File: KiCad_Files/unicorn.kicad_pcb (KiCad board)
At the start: 2 copper layers, 50 x 49.9 mm, 8 parts, among them SW1 SW_DIP_x01

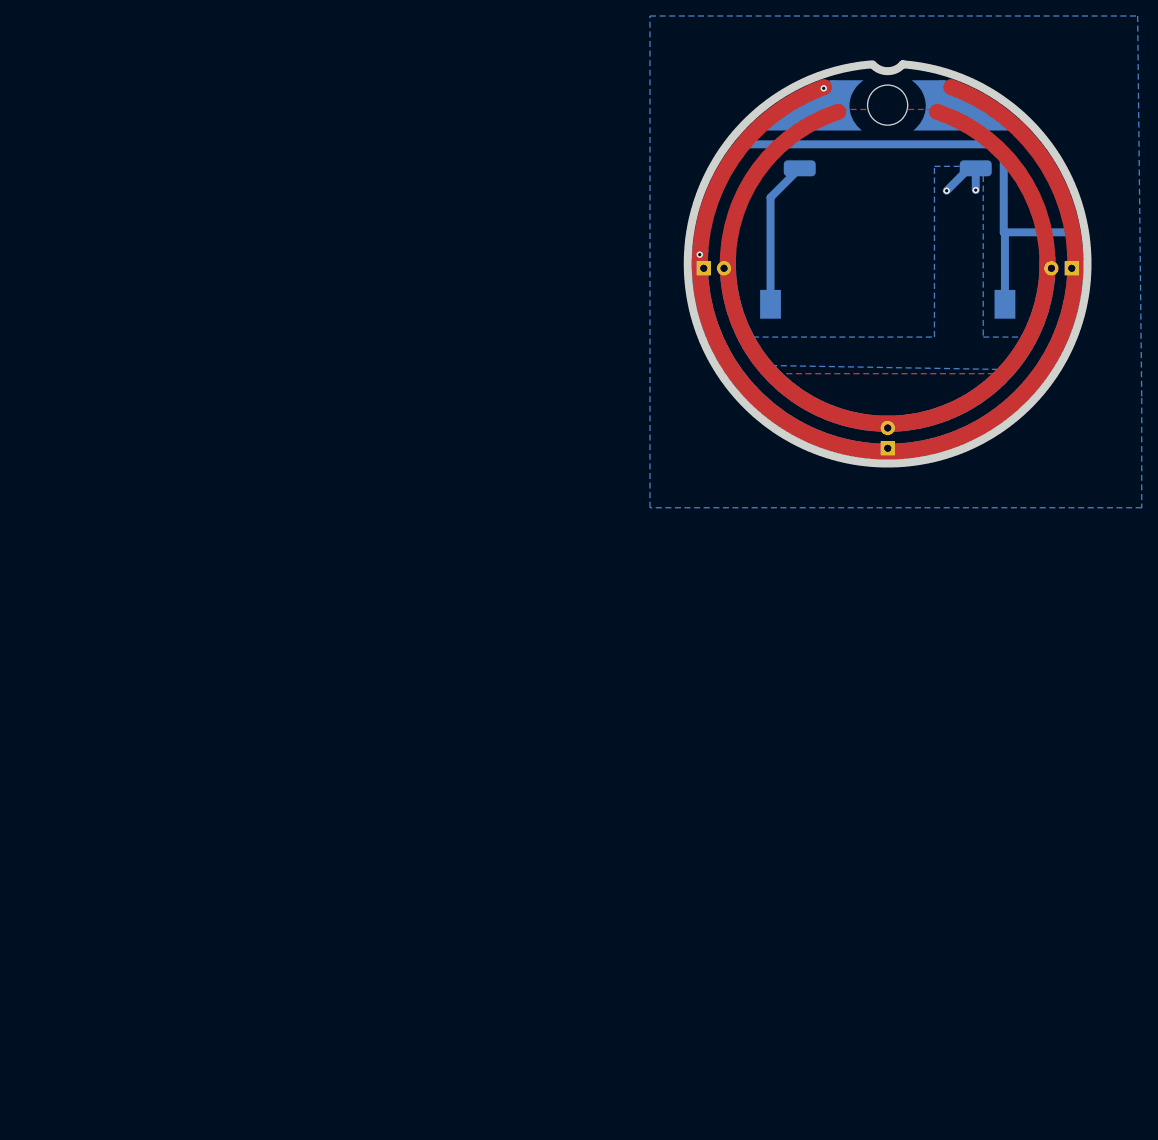
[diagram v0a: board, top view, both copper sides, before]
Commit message: kicad 0.5
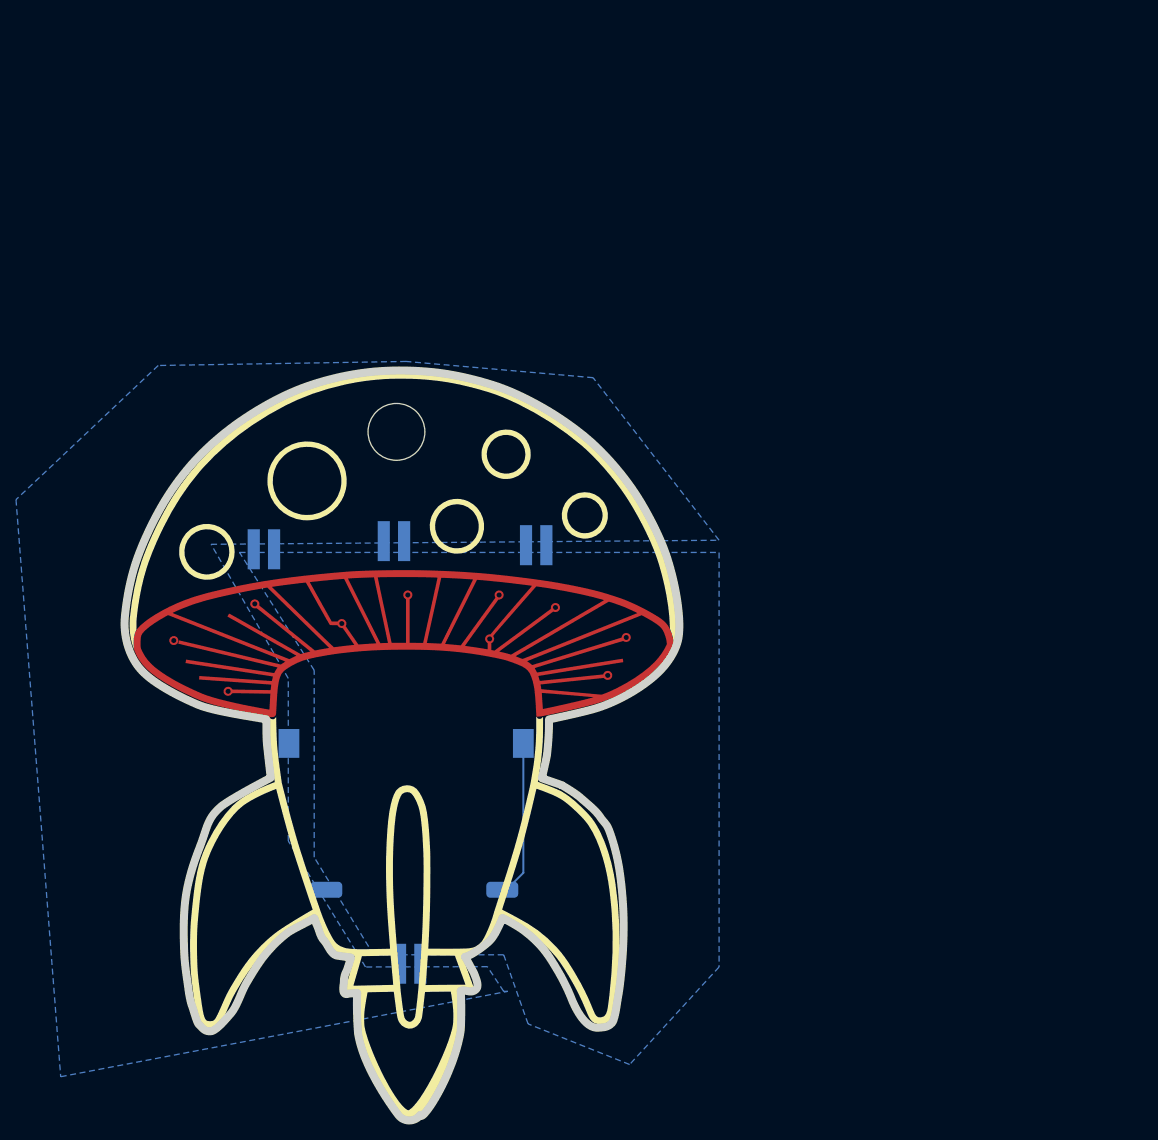
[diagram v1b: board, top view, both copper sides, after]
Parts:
- removed D1, D2, D3: LED, LED_THT:LED_D5.0mm_Clear
- removed the G*** at (91.0, 84.5)
- removed the REF** at (111.0, 93.0)
- added REF**: mushyrocket 0.5, blinkyparts:mushyrocket 0.5, F.Cu at (50.8, 151.9)
- added REF**: 5mm_SMD-Pad, blinkyparts:5mm_SMD-Pad, B.Cu at (33.3, 123.1)
- added REF**: 5mm_SMD-Pad, blinkyparts:5mm_SMD-Pad, B.Cu at (49.5, 122.1)
- added REF**: 5mm_SMD-Pad, blinkyparts:5mm_SMD-Pad, B.Cu at (67.3, 122.6)
- added REF**: 5mm_SMD-Pad, blinkyparts:5mm_SMD-Pad, B.Cu at (51.6, 174.9)
- moved SW1 122.7 mm to (39.8, 170.2), turned to 0 degrees
- moved G*** 110.5 mm to (74.7, 179.3)
- moved BT1 81.5 mm to (50.8, 151.9), turned to 180 degrees
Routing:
- net GND: track 78.4 -> 0.00 mm, vias 2 -> 0
- net VCC: track 7.52 -> 0.00 mm, vias 2 -> 0
- net +3V0: track 18.5 -> 20.4 mm
- removed copper zone on F.Cu, net VCC
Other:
- board size 50 x 49.9 mm -> 69.3 x 93.7 mm
- board text removed: "+"
- board text removed: "-"
- board text removed: "- - - - - -"
- board text removed: "area not connected"
